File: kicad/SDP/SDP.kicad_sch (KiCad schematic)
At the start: 82 parts, among them J1 GPIO, J2 SPI, J24 POWER, J25 Conn_01x04, J3 UART, J4 I2C, J5 Conn_01x04, J6 Conn_01x04, J7 RJ25, SW1 SW_Push_Dual, U1 TPS54233, U2 TPS54233, U3 PIC24FJ128GA010-I/PT, U4 DS3231SN-T&R, Y1 8MHz, Y2 32.768kHz

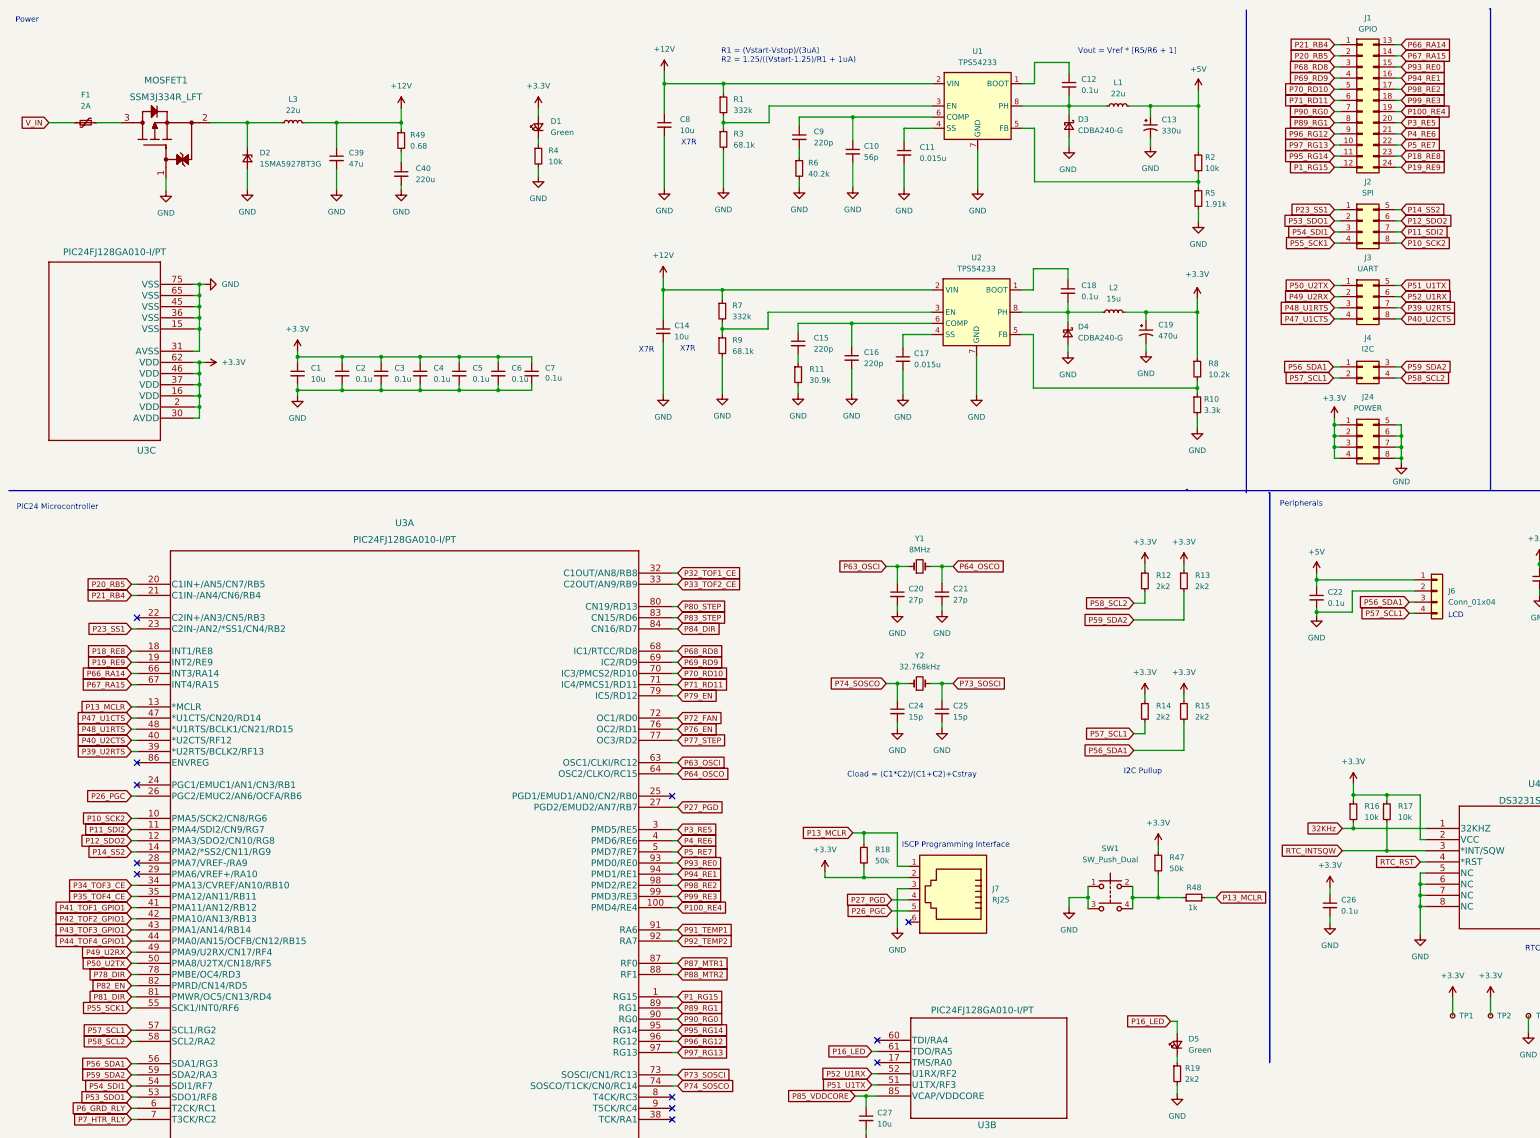
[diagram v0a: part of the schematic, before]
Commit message: PCB layout and schematic updates
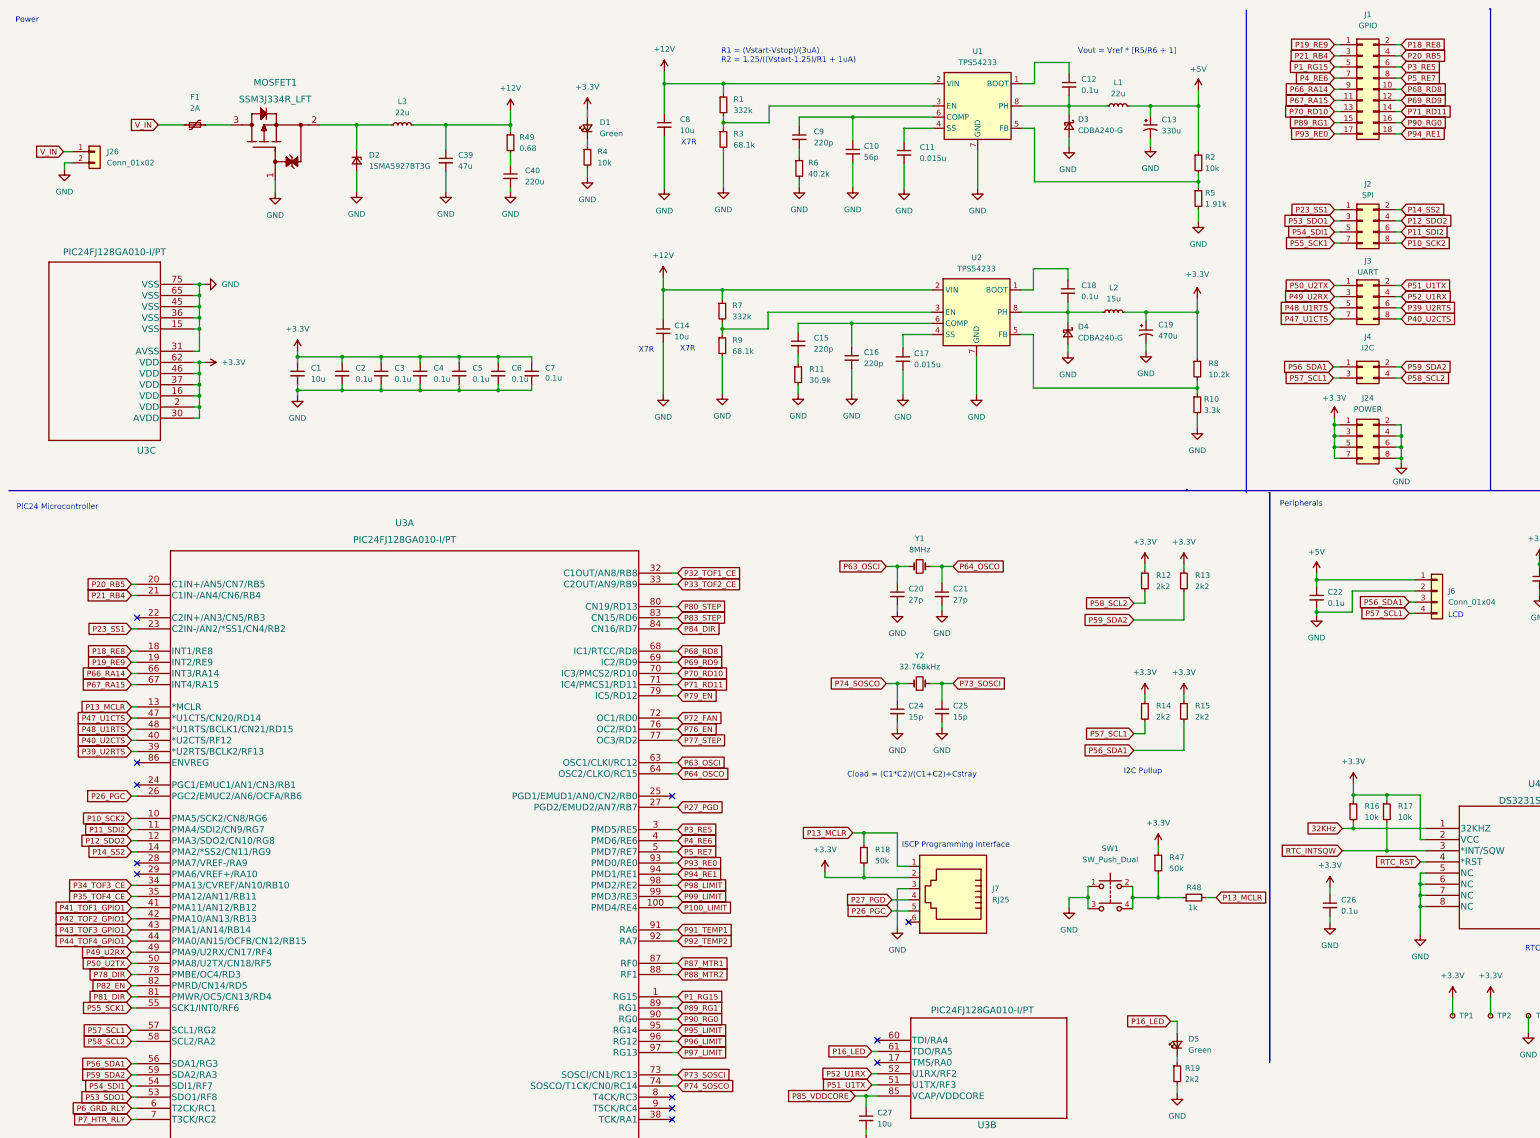
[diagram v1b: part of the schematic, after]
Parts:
- removed J1: GPIO, Connector_PinSocket_2.54mm:PinSocket_2x12_P2.54mm_Vertical, symbol Connector_Generic:Conn_02x12_Top_Bottom
- removed J2: SPI, Connector_PinSocket_2.54mm:PinSocket_2x04_P2.54mm_Vertical, symbol Connector_Generic:Conn_02x04_Top_Bottom
- removed J24: POWER, Connector_PinSocket_2.54mm:PinSocket_2x04_P2.54mm_Vertical, symbol Connector_Generic:Conn_02x04_Top_Bottom
- removed J3: UART, Connector_PinSocket_2.54mm:PinSocket_2x04_P2.54mm_Vertical, symbol Connector_Generic:Conn_02x04_Top_Bottom
- removed J4: I2C, Connector_PinSocket_2.54mm:PinSocket_2x02_P2.54mm_Vertical, symbol Connector_Generic:Conn_02x02_Top_Bottom
- added J1: GPIO, Connector_PinSocket_2.54mm:PinSocket_2x09_P2.54mm_Vertical, symbol Connector_Generic:Conn_02x09_Odd_Even
- added J2: SPI, Connector_PinSocket_2.54mm:PinSocket_2x04_P2.54mm_Vertical, symbol Connector_Generic:Conn_02x04_Odd_Even
- added J24: POWER, Connector_PinSocket_2.54mm:PinSocket_2x04_P2.54mm_Vertical, symbol Connector_Generic:Conn_02x04_Odd_Even
- added J26: Conn_01x02, TerminalBlock_Phoenix:TerminalBlock_Phoenix_PT-1,5-2-5.0-H_1x02_P5.00mm_Horizontal, symbol Connector_Generic:Conn_01x02
- added J3: UART, Connector_PinSocket_2.54mm:PinSocket_2x04_P2.54mm_Vertical, symbol Connector_Generic:Conn_02x04_Odd_Even
- added J4: I2C, Connector_PinSocket_2.54mm:PinSocket_2x02_P2.54mm_Vertical, symbol Connector_Generic:Conn_02x02_Odd_Even
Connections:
- net +3V3: now also J24.1 (Pin_1), J24.3 (Pin_3), J24.5 (Pin_5), J24.7 (Pin_7)
- net GND: now also J24.2 (Pin_2), J24.4 (Pin_4), J24.6 (Pin_6), J24.8 (Pin_8), J26.2 (Pin_2)
- net P10_SCK2: now also J2.8 (Pin_8)
- net P11_SDI2: now also J2.6 (Pin_6)
- net P12_SDO2: now also J2.4 (Pin_4)
- net P14_SS2: now also J2.2 (Pin_2)
- net P18_RE8: now also J1.2 (Pin_2)
- net P19_RE9: now also J1.1 (Pin_1)
- net P1_RG15: now also J1.5 (Pin_5)
- net P20_RB5: now also J1.4 (Pin_4)
- net P21_RB4: now also J1.3 (Pin_3)
- net P23_SS1: now also J2.1 (Pin_1)
- net P39_U2RTS: now also J3.6 (Pin_6)
- net P3_RE5: now also J1.6 (Pin_6)
- net P40_U2CTS: now also J3.8 (Pin_8)
- net P47_U1CTS: now also J3.7 (Pin_7)
- net P48_U1RTS: now also J3.5 (Pin_5)
- net P49_U2RX: now also J3.3 (Pin_3)
- net P4_RE6: now also J1.7 (Pin_7)
- net P50_U2TX: now also J3.1 (Pin_1)
- net P51_U1TX: now also J3.2 (Pin_2)
- net P52_U1RX: now also J3.4 (Pin_4)
- net P53_SDO1: now also J2.3 (Pin_3)
- net P54_SDI1: now also J2.5 (Pin_5)
- net P55_SCK1: now also J2.7 (Pin_7)
- net P56_SDA1: now also J4.1 (Pin_1)
- net P57_SCL1: now also J4.3 (Pin_3)
- net P58_SCL2: now also J4.4 (Pin_4)
- net P59_SDA2: now also J4.2 (Pin_2)
- net P5_RE7: now also J1.8 (Pin_8)
- net P66_RA14: now also J1.9 (Pin_9)
- net P67_RA15: now also J1.11 (Pin_11)
- net P68_RD8: now also J1.10 (Pin_10)
- net P69_RD9: now also J1.12 (Pin_12)
- net P70_RD10: now also J1.13 (Pin_13)
- net P71_RD11: now also J1.14 (Pin_14)
- net P89_RG1: now also J1.15 (Pin_15)
- net P90_RG0: now also J1.16 (Pin_16)
- net P93_RE0: now also J1.17 (Pin_17)
- net P94_RE1: now also J1.18 (Pin_18)
- net V_IN: now also J26.1 (Pin_1)
- net P100_RE4 renamed P100_LIMIT
- net P95_RG14 renamed P95_LIMIT
- net P96_RG12 renamed P96_LIMIT
- net P97_RG13 renamed P97_LIMIT
- net P98_RE2 renamed P98_LIMIT
- net P99_RE3 renamed P99_LIMIT
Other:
- moved on the sheet: C39, C40, D1, D2, F1, L3, MOSFET1, R4, R49
